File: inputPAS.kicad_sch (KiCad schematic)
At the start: 10 parts

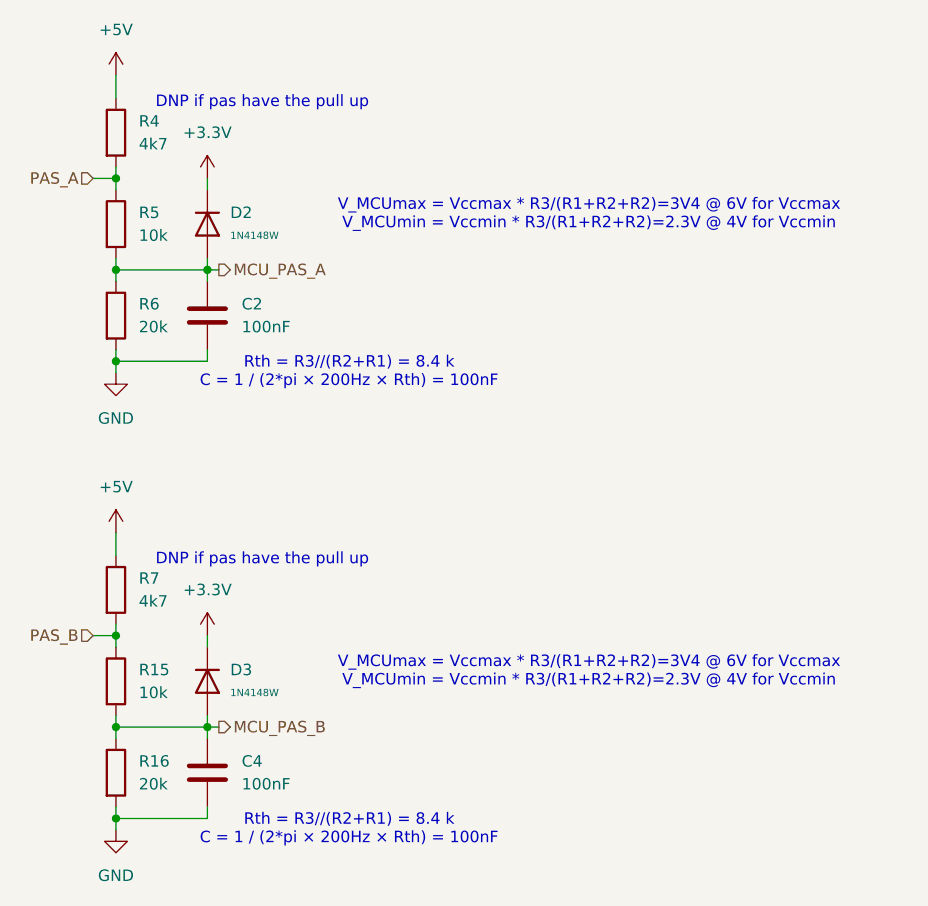
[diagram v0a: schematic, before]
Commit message: started pin assignement
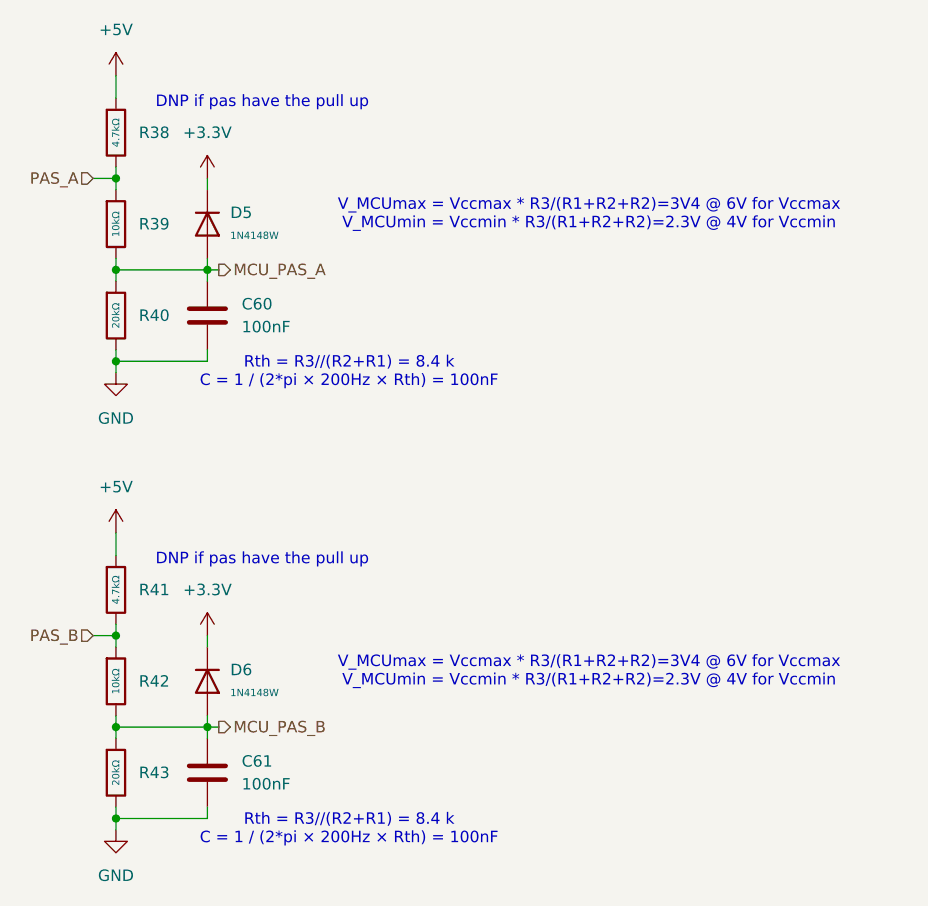
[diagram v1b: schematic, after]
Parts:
- removed R15, R5: 10k, symbol Device:R
- removed R16, R6: 20k, symbol Device:R
- removed R4, R7: 4k7, symbol Device:R
- added R38, R41: 4.7kΩ, PCM_JLCPCB:R_0805, symbol PCM_JLCPCB-Resistors:0805,4.7kΩ
- added R39, R42: 10kΩ, PCM_JLCPCB:R_0805, symbol PCM_JLCPCB-Resistors:0805,10kΩ
- added R40, R43: 20kΩ, PCM_JLCPCB:R_0805, symbol PCM_JLCPCB-Resistors:0805,20kΩ
- renumbered C2 to C60, C4 to C61, D2 to D5, D3 to D6
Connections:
- net +5V: now also R38.1, R41.1
- net GND: now also R40.2, R43.2
- net MCU_PAS_A: now also R39.2, R40.1
- net MCU_PAS_B: now also R42.2, R43.1
- net PAS_A: now also R38.2, R39.1
- net PAS_B: now also R41.2, R42.1
